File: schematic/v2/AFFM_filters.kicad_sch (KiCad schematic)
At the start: 24 parts, among them K1 DIPxx-1Axx-11x, K2 DIPxx-1Axx-11x, K3 DIPxx-1Axx-11x, K4 DIPxx-1Axx-11x

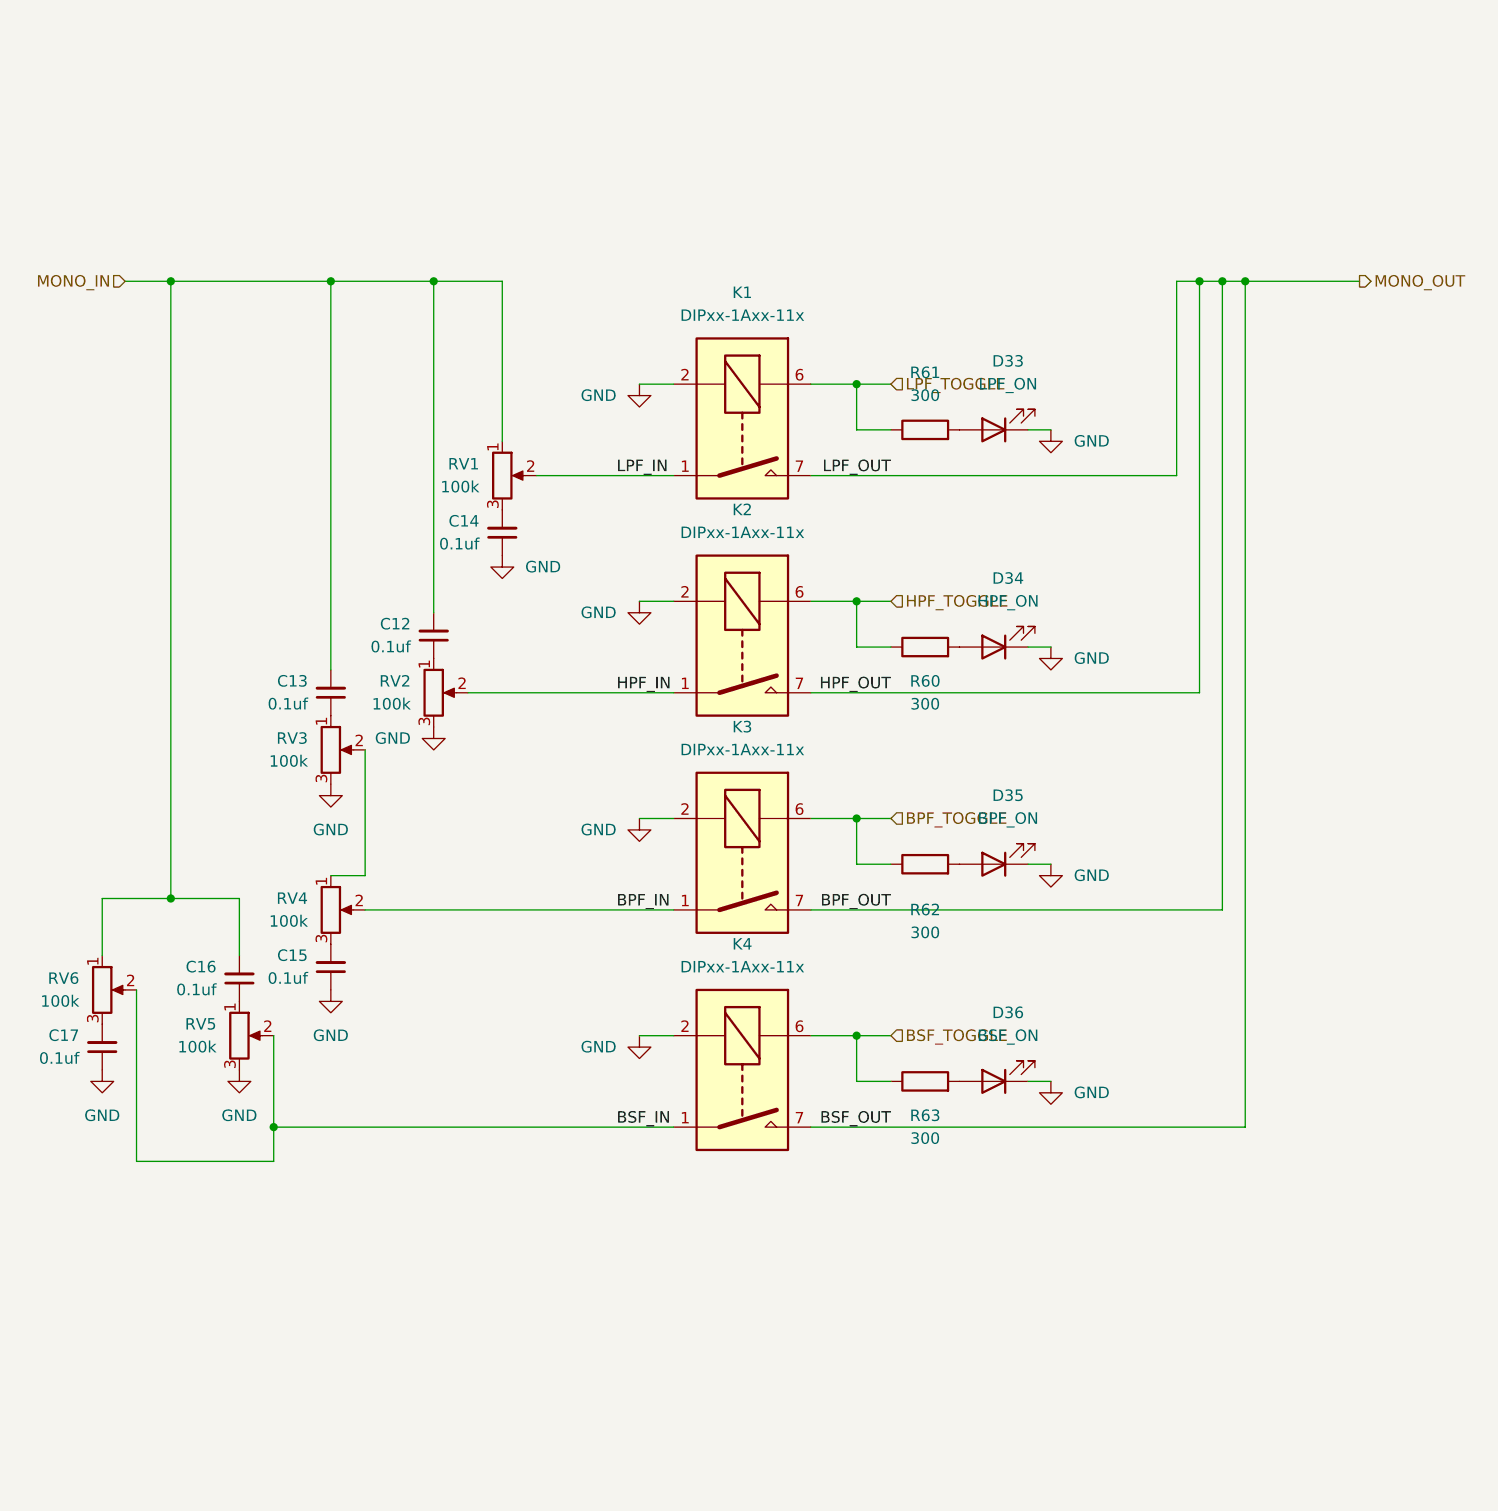
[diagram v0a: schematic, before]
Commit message: dip switch symbol. how might this work...
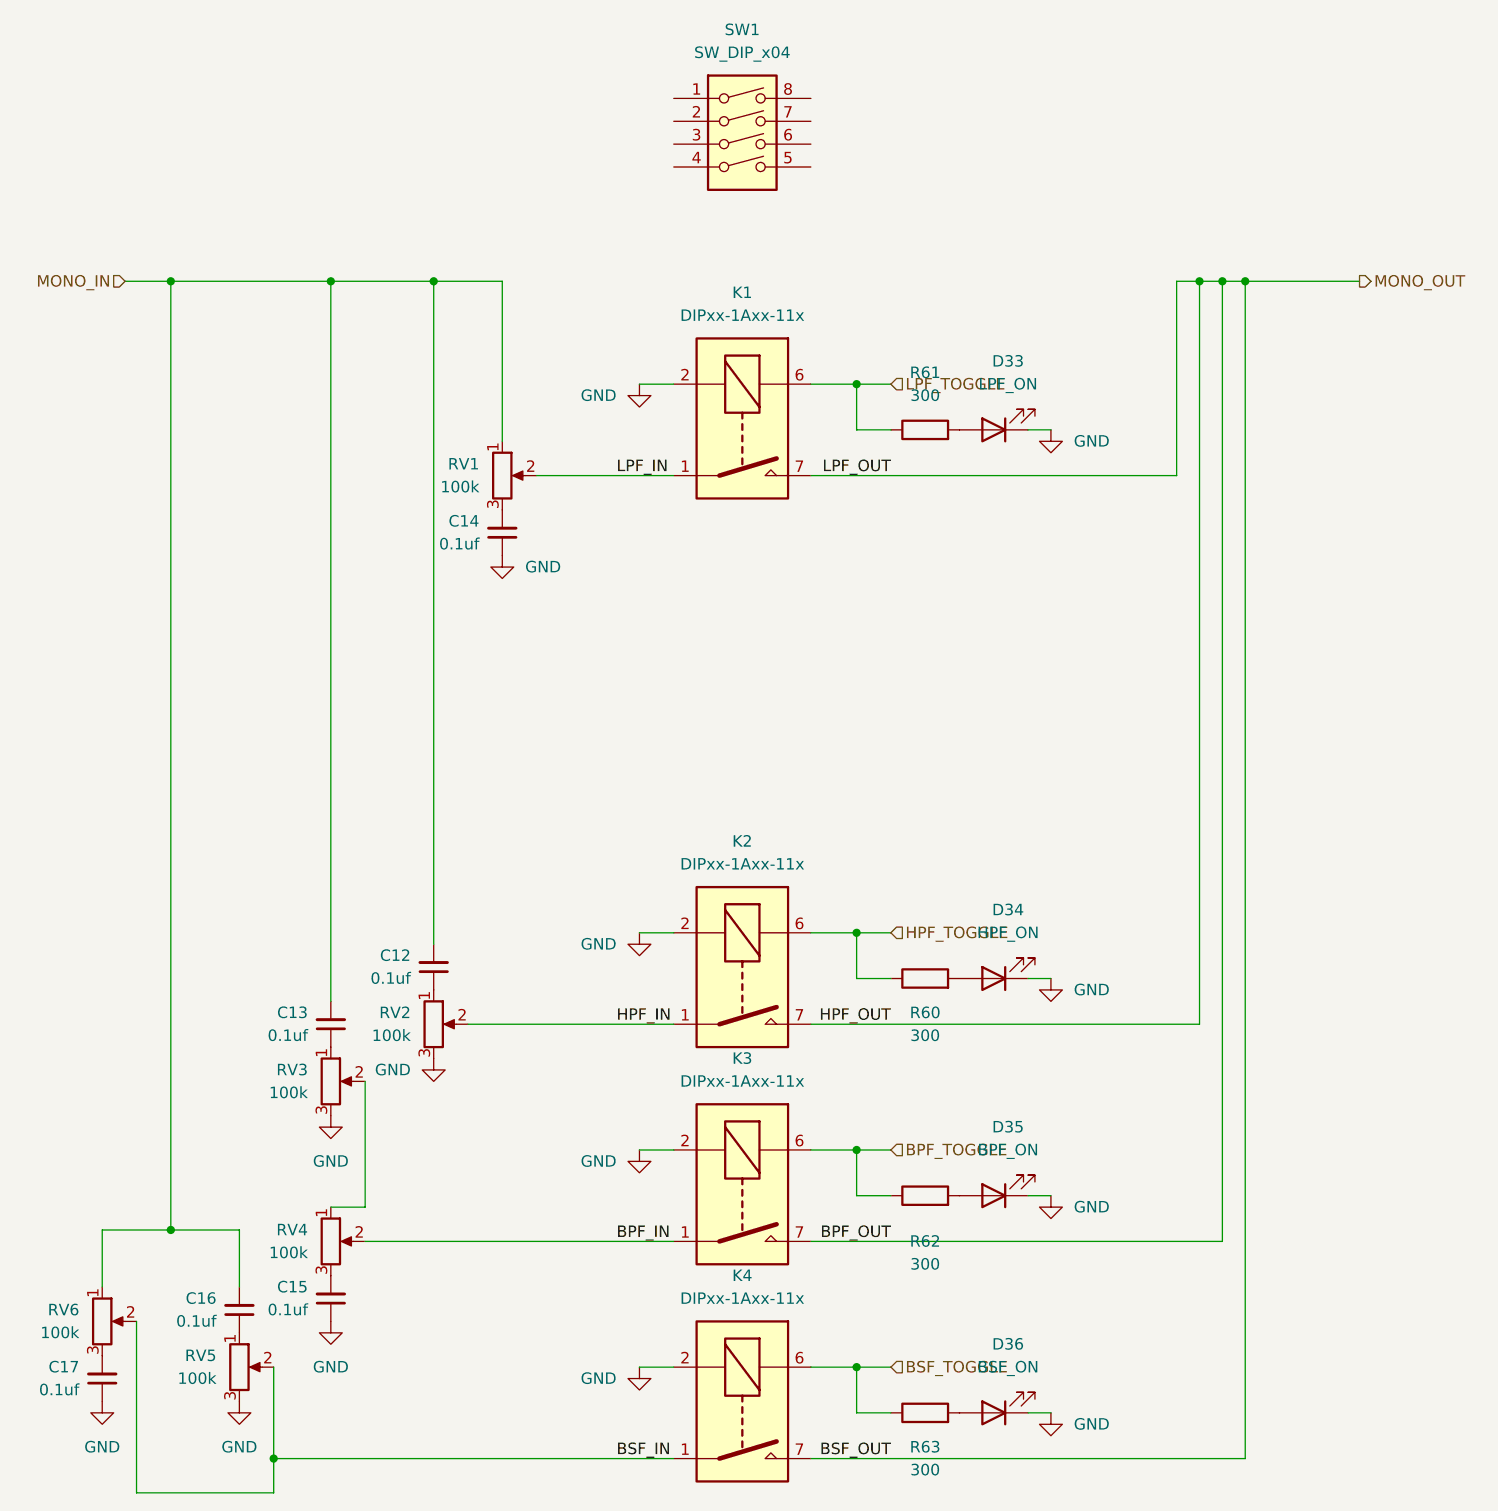
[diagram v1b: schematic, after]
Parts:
- added SW1: SW_DIP_x04, symbol Switch:SW_DIP_x04
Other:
- moved on the sheet: C12, C13, C15, C16, C17, D34, D35, D36, K2, K3, K4, R60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
